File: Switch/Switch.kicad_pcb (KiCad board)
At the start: 2 copper layers, 76.3 x 128.5 mm, 63 parts, among them J1 Conn_01x14_Pin, J2 Conn_01x14_Pin, J3 Conn_01x06_Pin, Q1 BC547, Q2 BC547, Q3 BC547, Q4 BC547, U1 TL074, U11 Aux_flush, U12 Aux_flush, U13 Aux_flush, U14 Aux_flush, U15 Aux_flush, U16 Aux_flush, U2 CD4066BE, U3 TL074, U4 Aux_flush, U5 Aux_flush, U6 Aux_flush, U7 Aux_flush, U8 Aux_flush, U9 Aux_flush

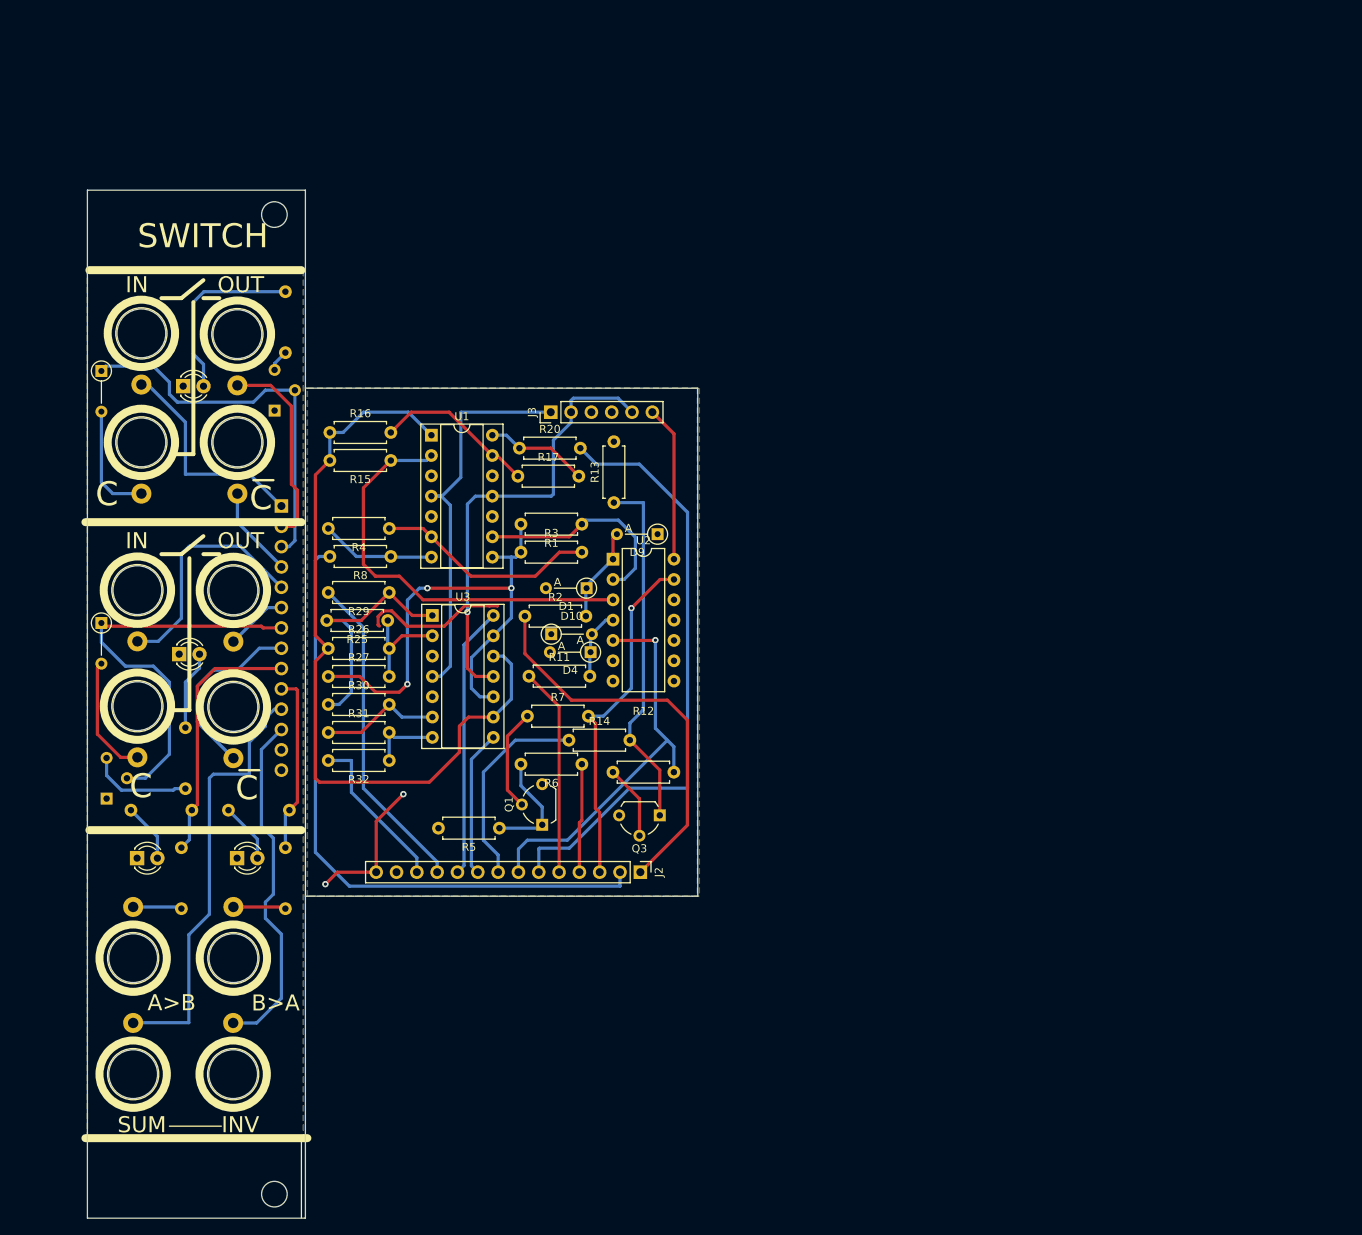
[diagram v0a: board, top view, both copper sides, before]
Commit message: Add files via upload
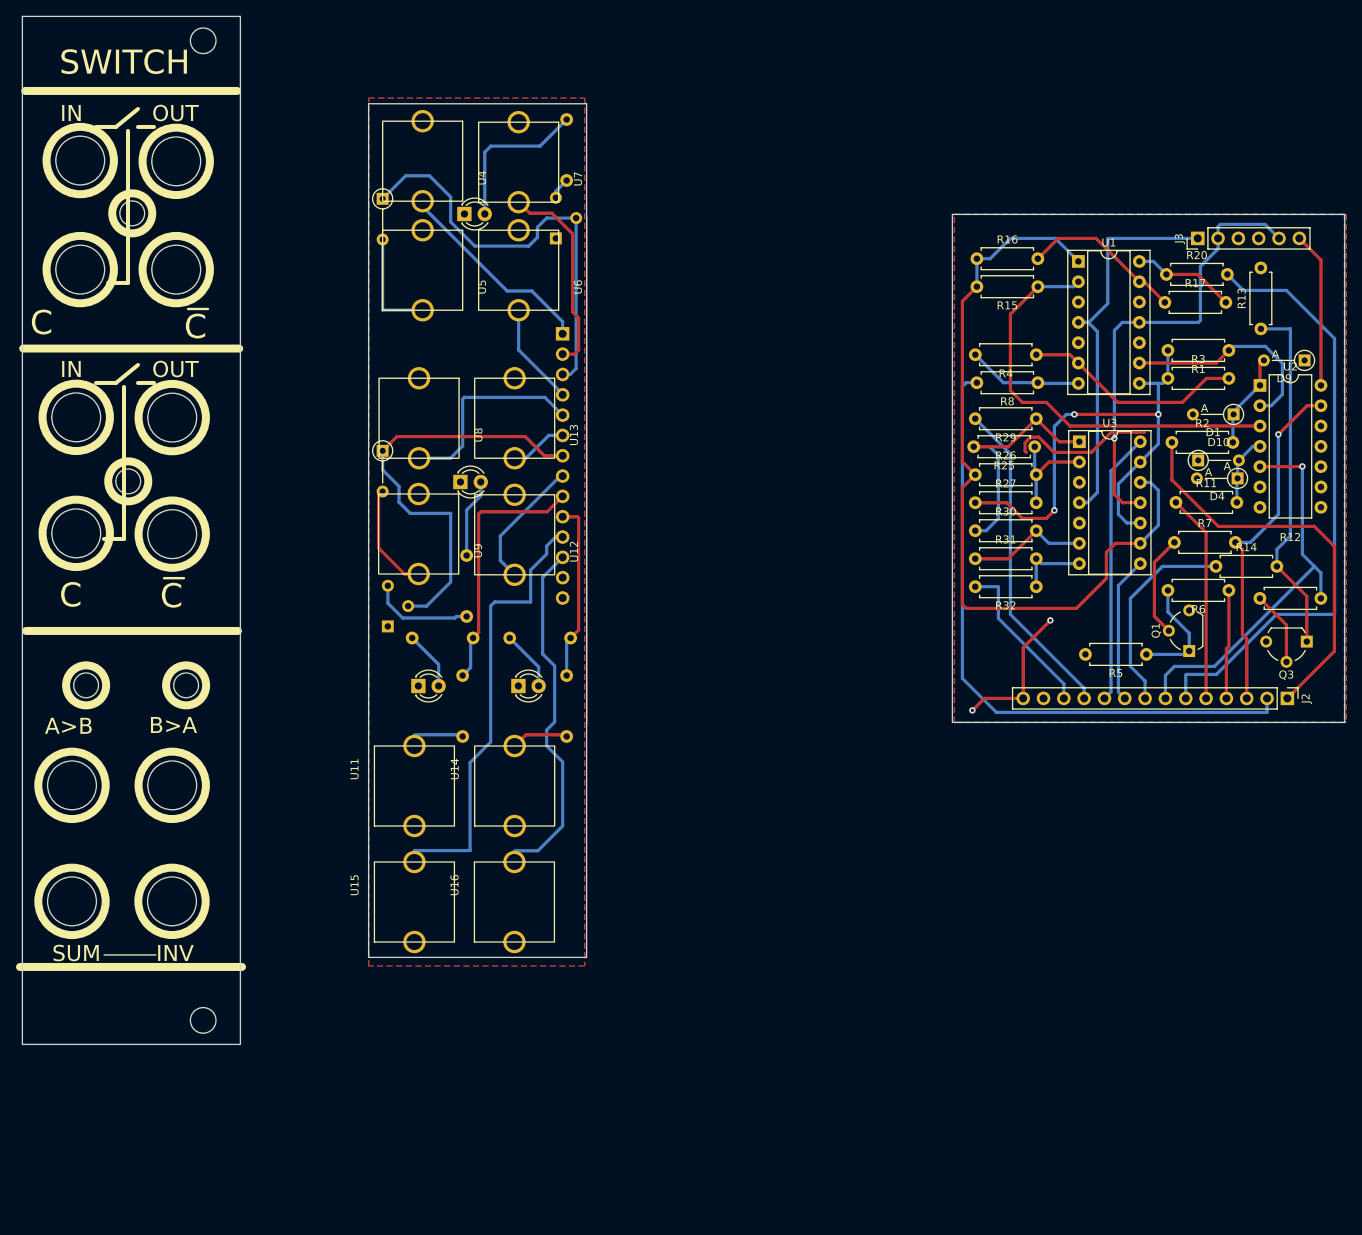
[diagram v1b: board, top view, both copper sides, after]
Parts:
- added ?: , , F.Cu at (65.2, 122.9)
- added ?: , , F.Cu at (65.2, 137.4)
- added ?: , , F.Cu at (66.2, 44.8)
- added ?: , , F.Cu at (77.7, 76.9)
- added ?: , , F.Cu at (72.2, 84.9)
- added ?: , , F.Cu at (77.7, 137.4)
- added ?: , , F.Cu at (78.2, 58.4)
- added ?: , , B.Cu at (65.7, 91.4)
- added ?: , , F.Cu at (78.2, 44.9)
- added ?: , , F.Cu at (79.5, 110.4)
- added ?: , , F.Cu at (72.7, 51.4)
- added ?: , , F.Cu at (65.7, 76.9)
- added ?: , , F.Cu at (67.0, 110.4)
- added ?: , , F.Cu at (77.7, 91.5)
- added ?: , , F.Cu at (66.2, 58.4)
- added ?: , , F.Cu at (77.7, 122.9)
- U11, U12, U13, U14, U15, U16, U4, U5, U6, U7, U8, U9: footprint Library:aux_flush -> Library:3mm5 Mono Aux
- moved R26 83.7 mm to (178.1, 84.1)
- moved R27 83.7 mm to (178.1, 87.6)
- moved R30 83.7 mm to (178.1, 91.1)
- moved R31 83.7 mm to (178.1, 94.6)
- moved R4 83.7 mm to (185.7, 69.1)
- moved D10 83.7 mm to (206.0, 82.3)
- moved R15 83.7 mm to (185.9, 60.6)
- moved R16 83.7 mm to (178.3, 57.1)
- moved R8 83.7 mm to (185.9, 72.6)
- moved U3 83.7 mm to (191.1, 79.9)
- moved D1 83.7 mm to (210.4, 76.5)
- moved D4 83.7 mm to (210.9, 84.5)
- moved D9 83.7 mm to (219.3, 69.8)
- moved J2 83.7 mm to (217.1, 112.0)
- moved Q1 83.7 mm to (204.8, 106.1)
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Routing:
- net INV2: track 48.9 -> 42.1 mm
- net C1: track 92.4 -> 97.7 mm
- net IN2: track 55.8 -> 51.5 mm
- net Net-(D3-A): track 23.1 -> 19.7 mm
- net C2: track 101.7 -> 104.1 mm
- net IN1: track 77.5 -> 75.5 mm
- net Net-(D5-A): track 15.2 -> 13.6 mm
- net Net-(D2-A): track 14.4 -> 13.8 mm
- net OUT2: track 83.6 -> 83.0 mm
- net OUT1: track 104.9 -> 105.5 mm
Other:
- board size 76.3 x 128.5 mm -> 165.3 x 128.5 mm
